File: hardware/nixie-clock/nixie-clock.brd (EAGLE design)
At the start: 100 x 80 mm, 0 parts

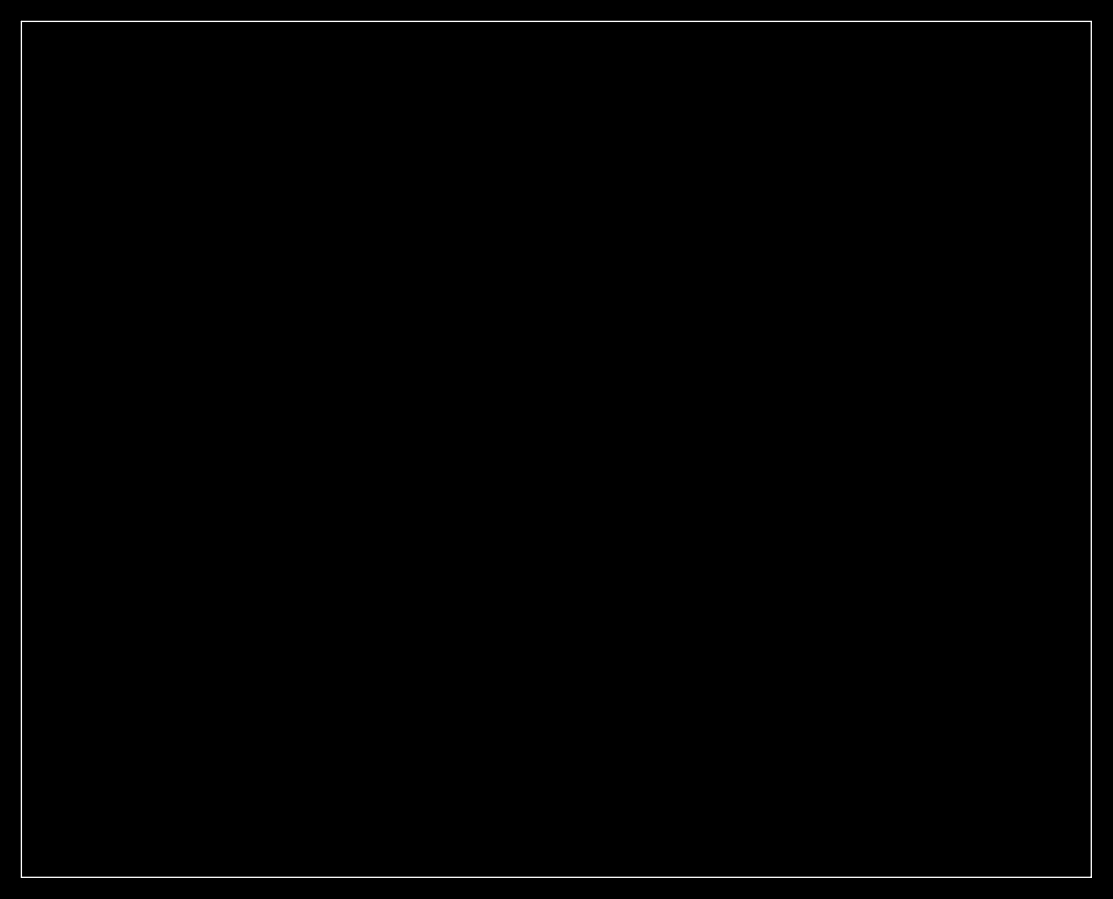
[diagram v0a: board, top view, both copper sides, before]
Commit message: Board design
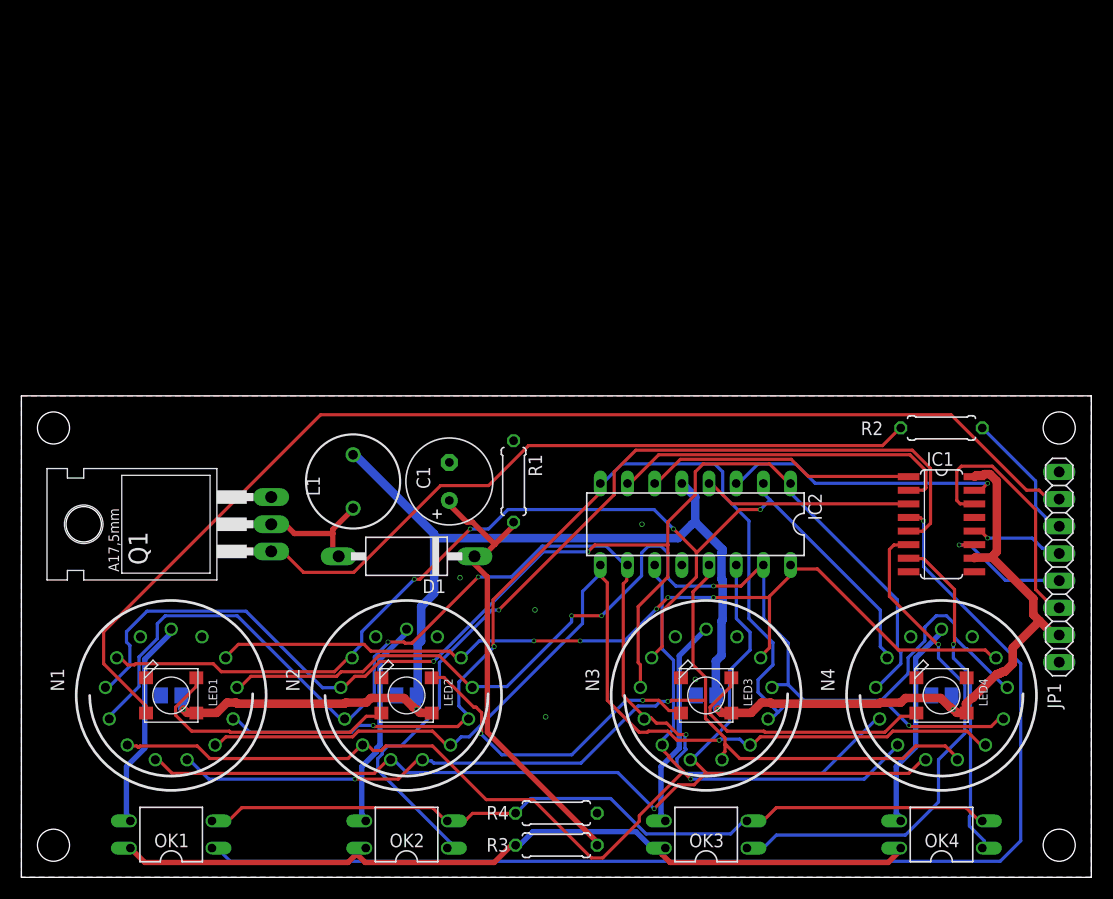
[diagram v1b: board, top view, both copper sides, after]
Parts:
- added C1: 4.7uF, rcl:E3,5-8
- added C2, C3, C4, C5: 0.1u, rcl:C0805
- added D1: HER106, diode:DO15-12
- added IC1: 74HC595D, 74xx-eu:SO16
- added IC2: 74141N, 74xx-eu:DIL16
- added JP1: (no value), pinhead:1X08
- added L1: 220uH, rcl:6000-XXXX-RC
- added LED1, LED2, LED3, LED4: WS2812B_5050N, WS2812B:WS2812B-NARROW
- added N1, N2, N3, N4: IN-14, russian-nixies:IN-14
- added OK1, OK2, OK3, OK4: TIL197, optocoupler:DIL04
- added Q1: IRF840, IRF840:TO220
- added R1: 330, rcl:0207/7
- added R2: 22, rcl:0207/7
- added R3: 10K, rcl:0207/7
- added R4: 470, rcl:0207/7
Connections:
- new net +UB: C1.+, D1.C, R1.2, R3.2
- new net CLK: IC1.11, JP1.4
- new net DIN: IC1.14, JP1.3
- new net GND: C1.-, C2.2, C3.2, C4.2, C5.2, IC1.13, IC1.8, IC2.12, JP1.1, JP1.8, LED1.3-GND, LED2.3-GND, LED3.3-GND, LED4.3-GND, Q1.3, R1.1, R4.2
- new net LED_IN: JP1.7, LED1.4-DIN
- new net N$1: Q1.1, R2.2
- new net N$10: IC2.8, N1.3, N2.3, N3.3, N4.3
- new net N$11: IC2.9, N1.4, N2.4, N3.4, N4.4
- new net N$12: IC2.13, N1.5, N2.5, N3.5, N4.5
- new net N$13: IC2.14, N1.6, N2.6, N3.6, N4.6
- new net N$14: IC2.11, N1.7, N2.7, N3.7, N4.7
- new net N$15: IC2.10, N1.8, N2.8, N3.8, N4.8
- new net N$16: IC2.1, N1.9, N2.9, N3.9, N4.9
- new net N$17: IC2.2, N1.0, N2.0, N3.0, N4.0
- new net N$18: OK1.4, OK2.4, OK3.4, OK4.4, R3.1
- new net N$19: OK1.2, OK2.2, OK3.2, OK4.2, R4.1
- new net N$2: D1.A, L1.2, Q1.2
- new net N$20: IC1.4, OK1.1
- new net N$21: LED1.2-DOUT, LED2.4-DIN
- new net N$22: IC1.6, OK3.1
- new net N$23: IC1.7, OK4.1
- new net N$24: IC1.15, IC2.3
- new net N$25: IC1.1, IC2.6
- new net N$26: IC1.2, IC2.7
- new net N$27: IC1.3, IC2.4
- new net N$28: IC1.5, OK2.1
- new net N$29: LED2.2-DOUT, LED3.4-DIN
- new net N$30: LED3.2-DOUT, LED4.4-DIN
- new net N$8: IC2.16, N1.1, N2.1, N3.1, N4.1
- new net N$9: IC2.15, N1.2, N2.2, N3.2, N4.2
- new net N1_ANODE: N1.A, OK1.3
- new net N2_ANODE: N2.A, OK2.3
- new net N3_ANODE: N3.A, OK3.3
- new net N4_ANODE: N4.A, OK4.3
- new net PWM: JP1.6, R2.1
- new net RCLK: IC1.12, JP1.5
- new net VCC: C2.1, C3.1, C4.1, C5.1, IC1.10, IC1.16, IC2.5, JP1.2, L1.1, LED1.1-VDD, LED2.1-VDD, LED3.1-VDD, LED4.1-VDD
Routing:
- net VCC: track 0.00 -> 161.2 mm, vias 0 -> 4
- net N$16: track 0.00 -> 123.3 mm, vias 0 -> 2
- net N$15: track 0.00 -> 113.3 mm, vias 0 -> 3
- net N$10: track 0.00 -> 113.0 mm, vias 0 -> 3
- net N$20: track 0.00 -> 112.1 mm, vias 0 -> 1
- net LED_IN: track 0.00 -> 110.2 mm
- net N$9: track 0.00 -> 106.0 mm, vias 0 -> 3
- net N$17: track 0.00 -> 105.3 mm, vias 0 -> 4
- net N$14: track 0.00 -> 104.5 mm, vias 0 -> 1
- net N$13: track 0.00 -> 100.2 mm, vias 0 -> 1
- net N$11: track 0.00 -> 97.5 mm, vias 0 -> 1
- net N$12: track 0.00 -> 96.2 mm, vias 0 -> 2
- net N$8: track 0.00 -> 87.1 mm, vias 0 -> 5
- net N$28: track 0.00 -> 87.0 mm, vias 0 -> 1
- net N$18: track 0.00 -> 78.2 mm
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- added copper zone on layer 1, net GND
- added copper zone on layer 16, net GND
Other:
- board size 100 x 80 mm -> 100 x 45 mm
- board text added: "+5V"
- board text added: "CLK"
- board text added: "DIN"
- board text added: "LED"
- board text added: "Nixie Clock"
- board text added: "PWM"
- board text added: "RCLK"
